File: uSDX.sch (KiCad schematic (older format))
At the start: 21 parts

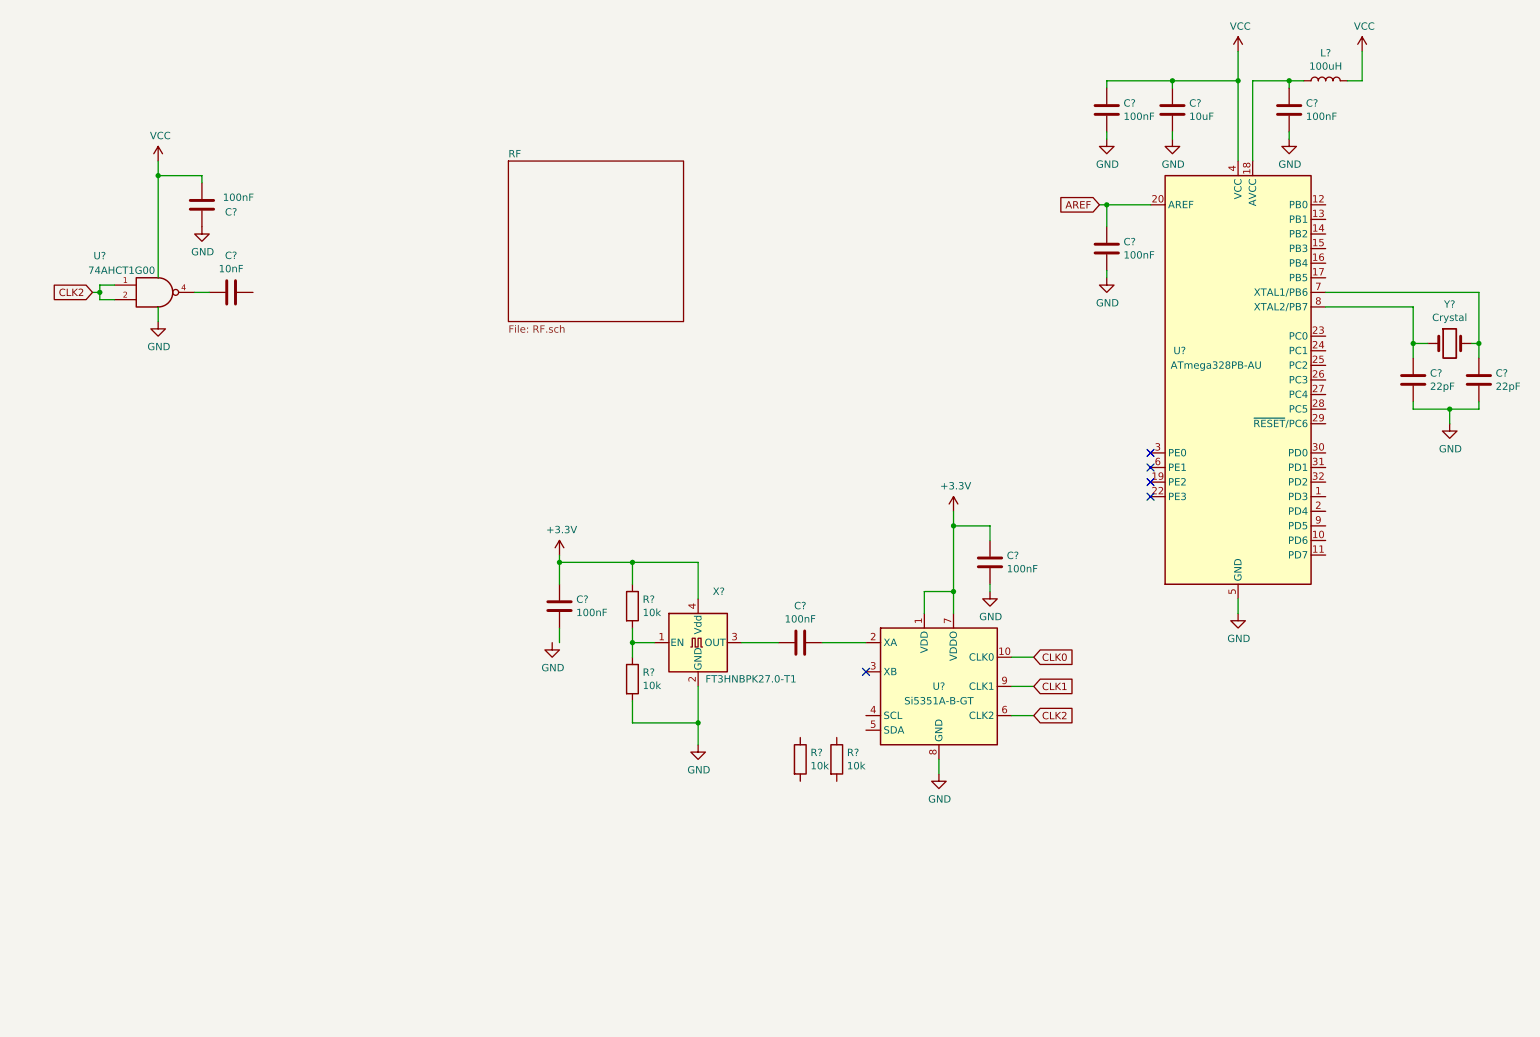
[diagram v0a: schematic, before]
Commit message: a
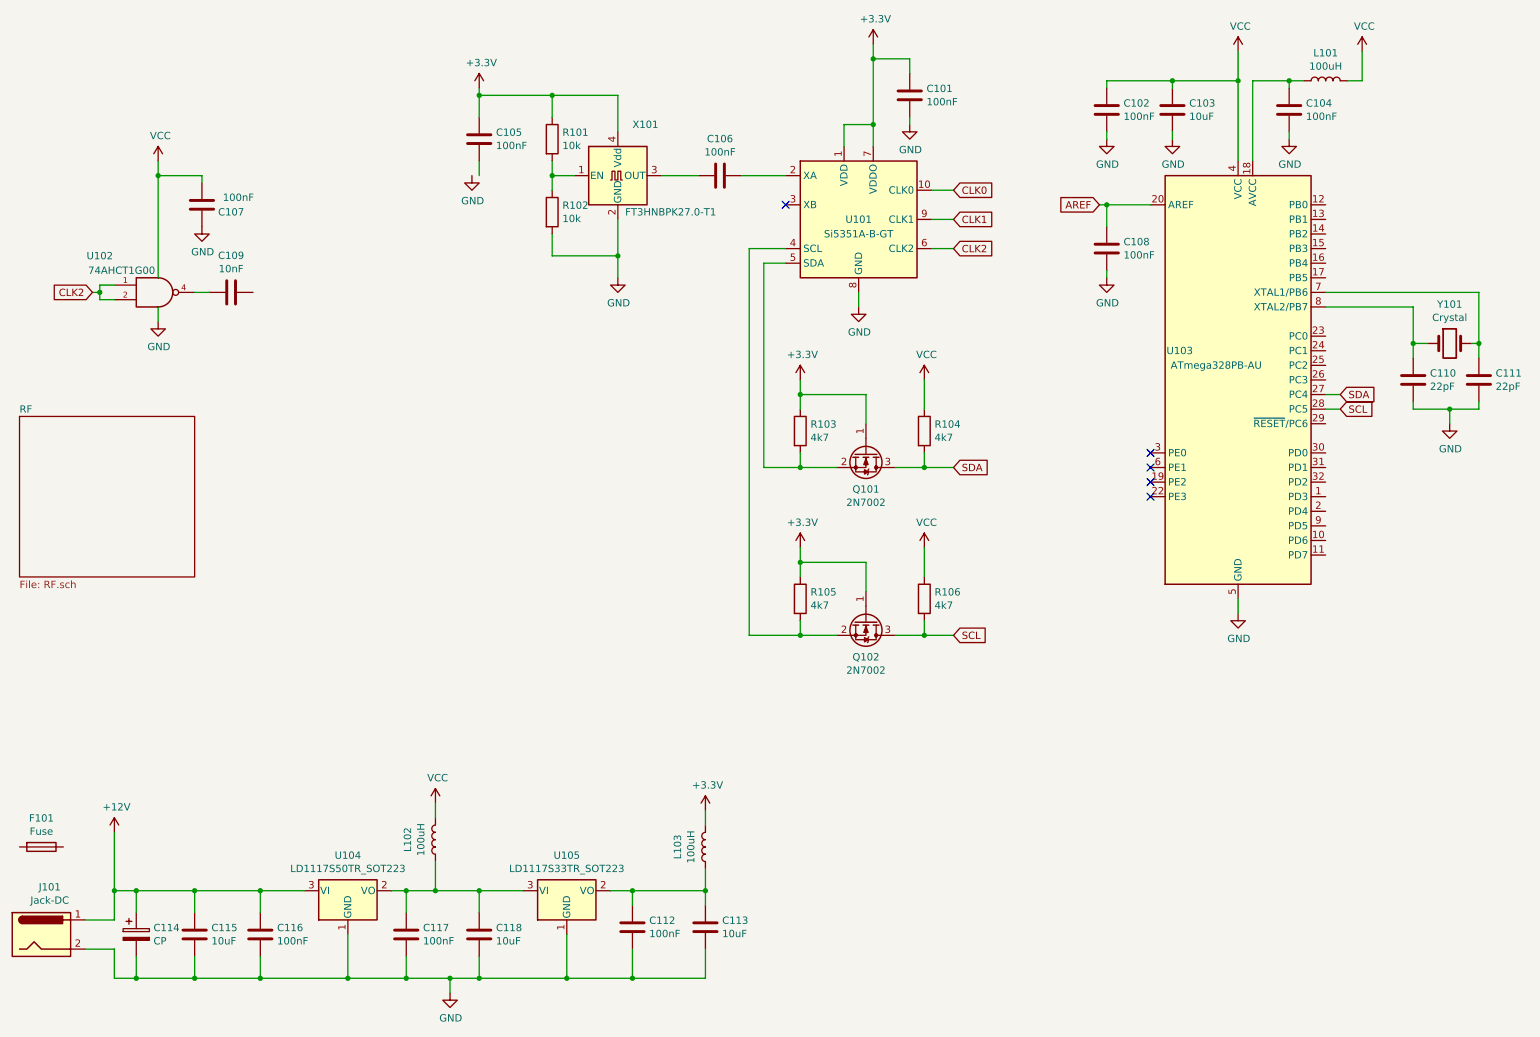
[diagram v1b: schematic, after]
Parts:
- removed R? (x2): 10k, symbol Device:R
- added C112, C116, C117: 100nF, symbol Device:C
- added C113, C115, C118: 10uF, symbol Device:C
- added C114: CP, symbol Device:CP
- added F101: Fuse, symbol Device:Fuse
- added J101: Jack-DC, symbol Connector:Jack-DC
- added L102, L103: 100uH, symbol Device:L
- added Q101, Q102: 2N7002, Package_TO_SOT_SMD:SOT-23, symbol Transistor_FET:2N7002
- added R103, R104, R105, R106: 4k7, symbol Device:R
- added U104: LD1117S50TR_SOT223, Package_TO_SOT_SMD:SOT-223-3_TabPin2, symbol Regulator_Linear:LD1117S50TR_SOT223
- added U105: LD1117S33TR_SOT223, Package_TO_SOT_SMD:SOT-223-3_TabPin2, symbol Regulator_Linear:LD1117S33TR_SOT223
- gave numbers to parts that had none: 19
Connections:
- net +3V3: now also L103.2, Q101.1 (G), Q102.1 (G), R103.1, R105.1
- net GND: now also C112.1, C113.1, C114.2, C115.1, C116.1, C117.1, C118.1, J101.2, U104.1 (GND), U105.1 (GND)
- net VCC: now also L102.2, R104.1, R106.1
- net SDA: now reaches U103.27 (PC4)
- net SDA: now also Q101.3 (D), R104.2
- net SCL: now reaches U103.28 (PC5)
- net SCL: now also Q102.3 (D), R106.2
- net at U101.4 (SCL): now also Q102.2 (S), R105.2
- net at U101.5 (SDA): now also Q101.2 (S), R103.2
- new net: C112.2, C113.2, L103.1, U105.2 (VO)
- new net: C117.2, C118.2, L102.1, U104.2 (VO), U105.3 (VI)
- new net +12V: C114.1, C115.2, C116.2, J101.1, U104.3 (VI)
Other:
- moved on the sheet: C101, C105, C106, R101, R102, U101, X101

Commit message: filter backup
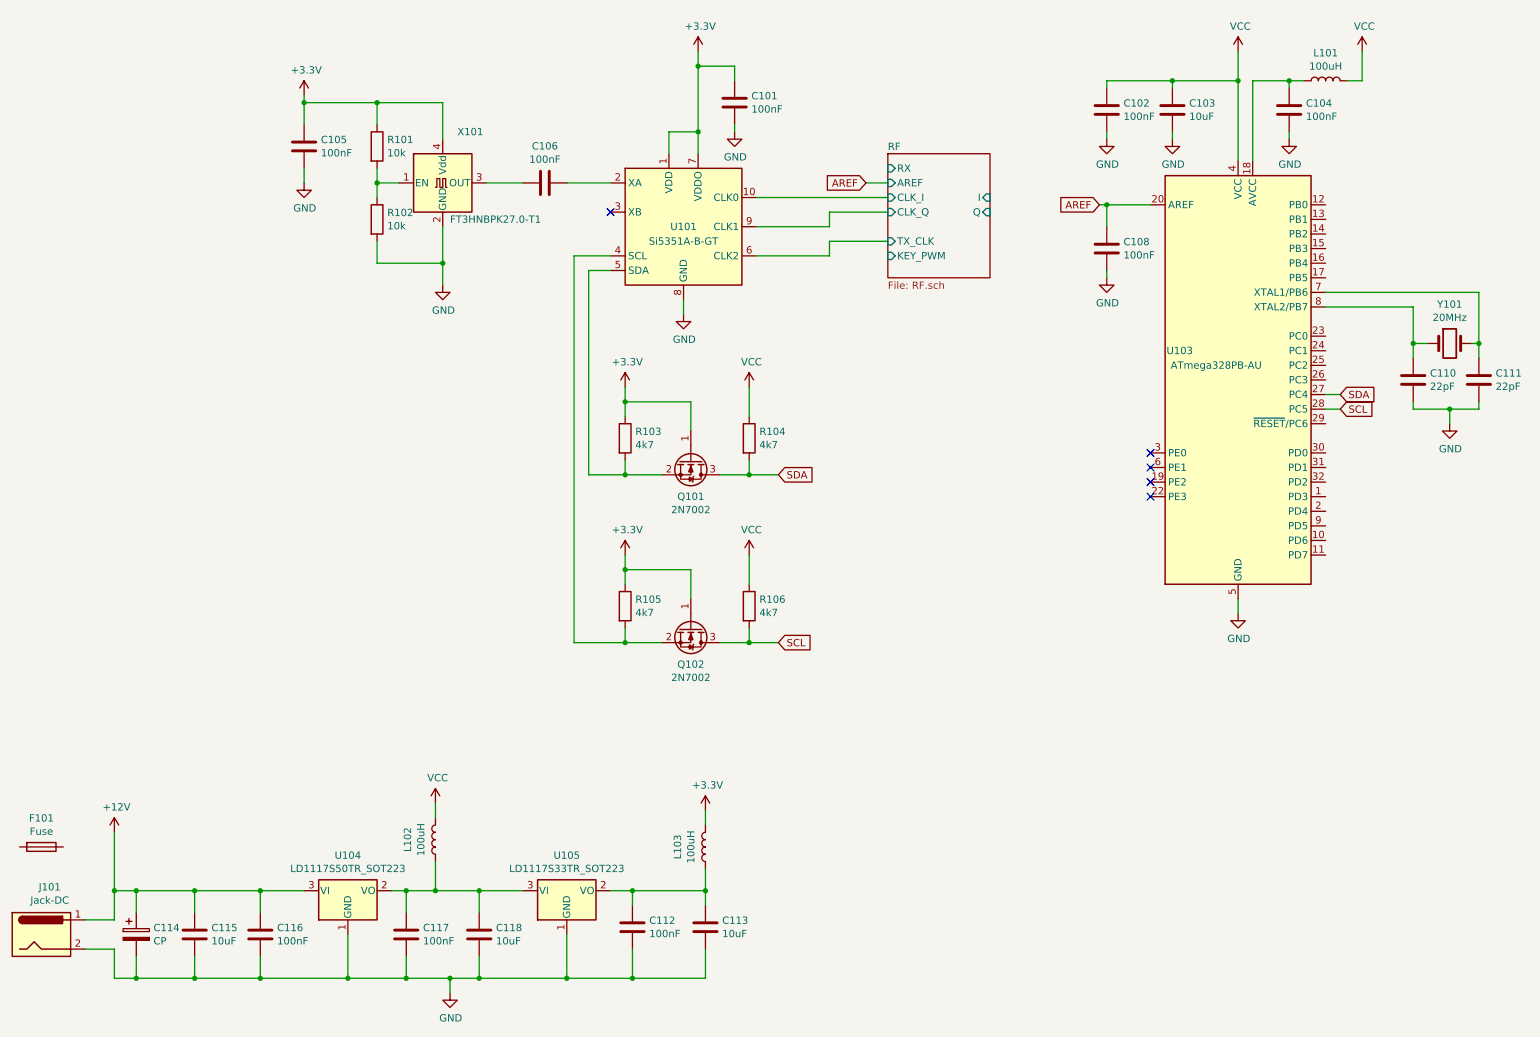
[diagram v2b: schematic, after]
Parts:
- removed C107: 100nF, symbol Device:C
- removed C109: 10nF, symbol Device:C
- removed U102: 74AHCT1G00, symbol 74xGxx:74AHCT1G00
- Y101: value Crystal -> 20MHz
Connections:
- net GND: now also C105.1
- net CLK0 renamed RF/CLK_I
- net CLK1 renamed RF/CLK_Q
- net CLK2 renamed RF/TX_CLK
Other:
- moved on the sheet: C101, C105, C106, Q101, Q102, R101, R102, R103, R104, R105, R106, U101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
